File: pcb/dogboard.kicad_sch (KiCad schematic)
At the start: 41 parts, among them J1 USB-C / USB2.0, SW2 Action, SW3 Action, U1 RP2040, U3 8MB Flash, Y1 12 MHz

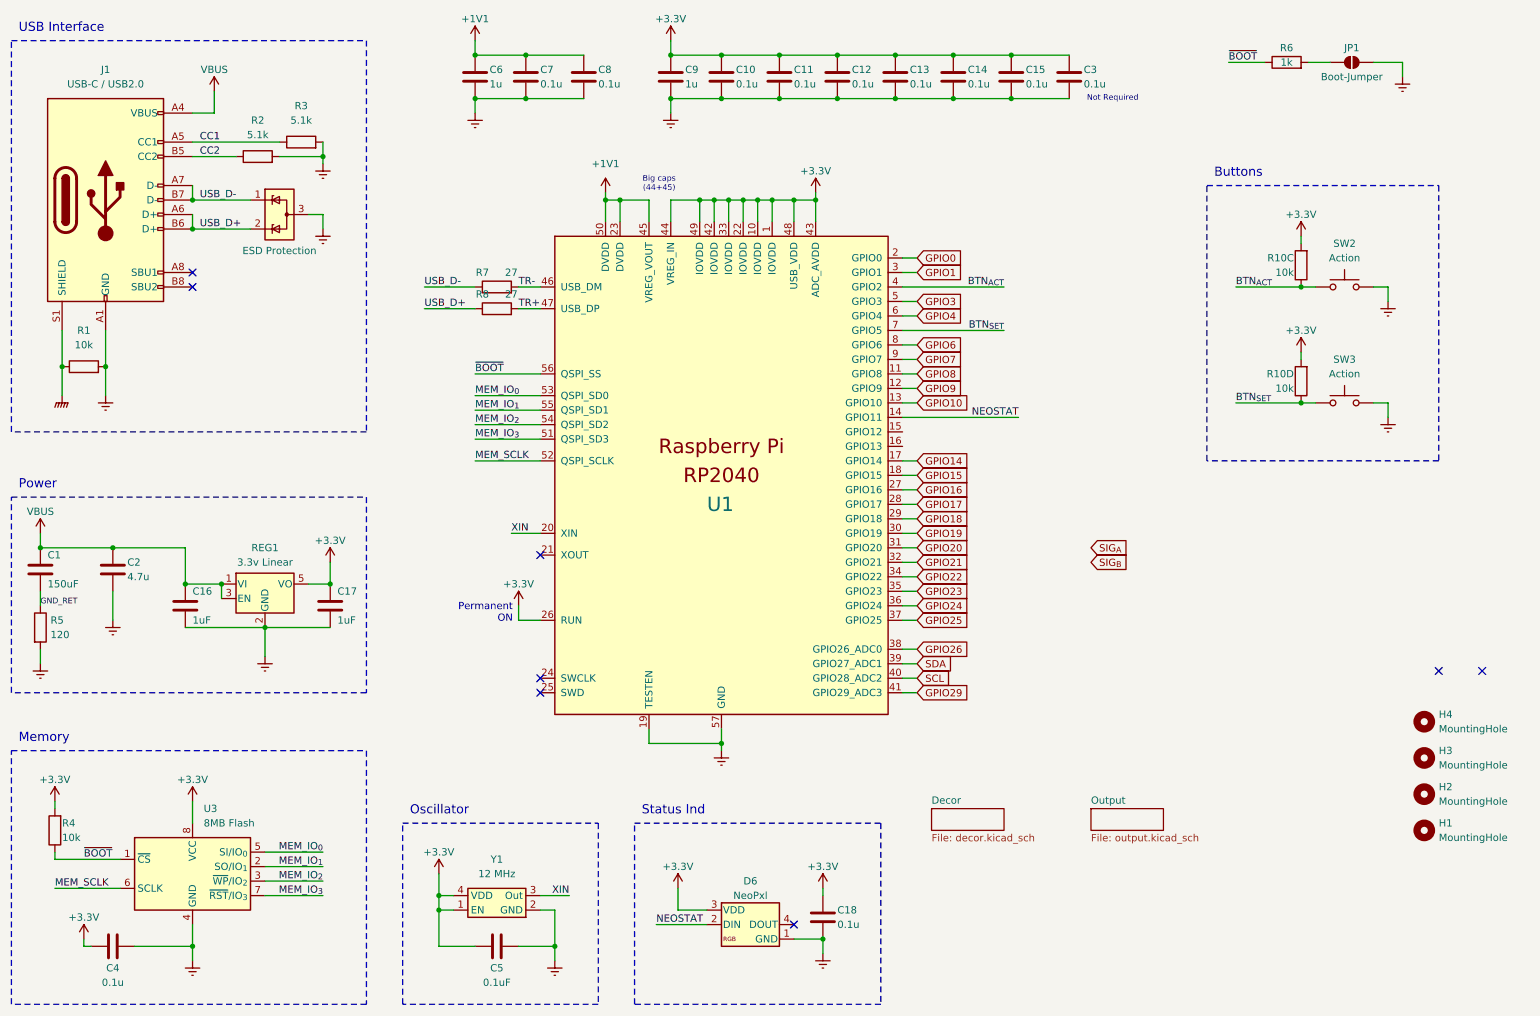
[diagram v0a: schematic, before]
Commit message: dogboard-2b4
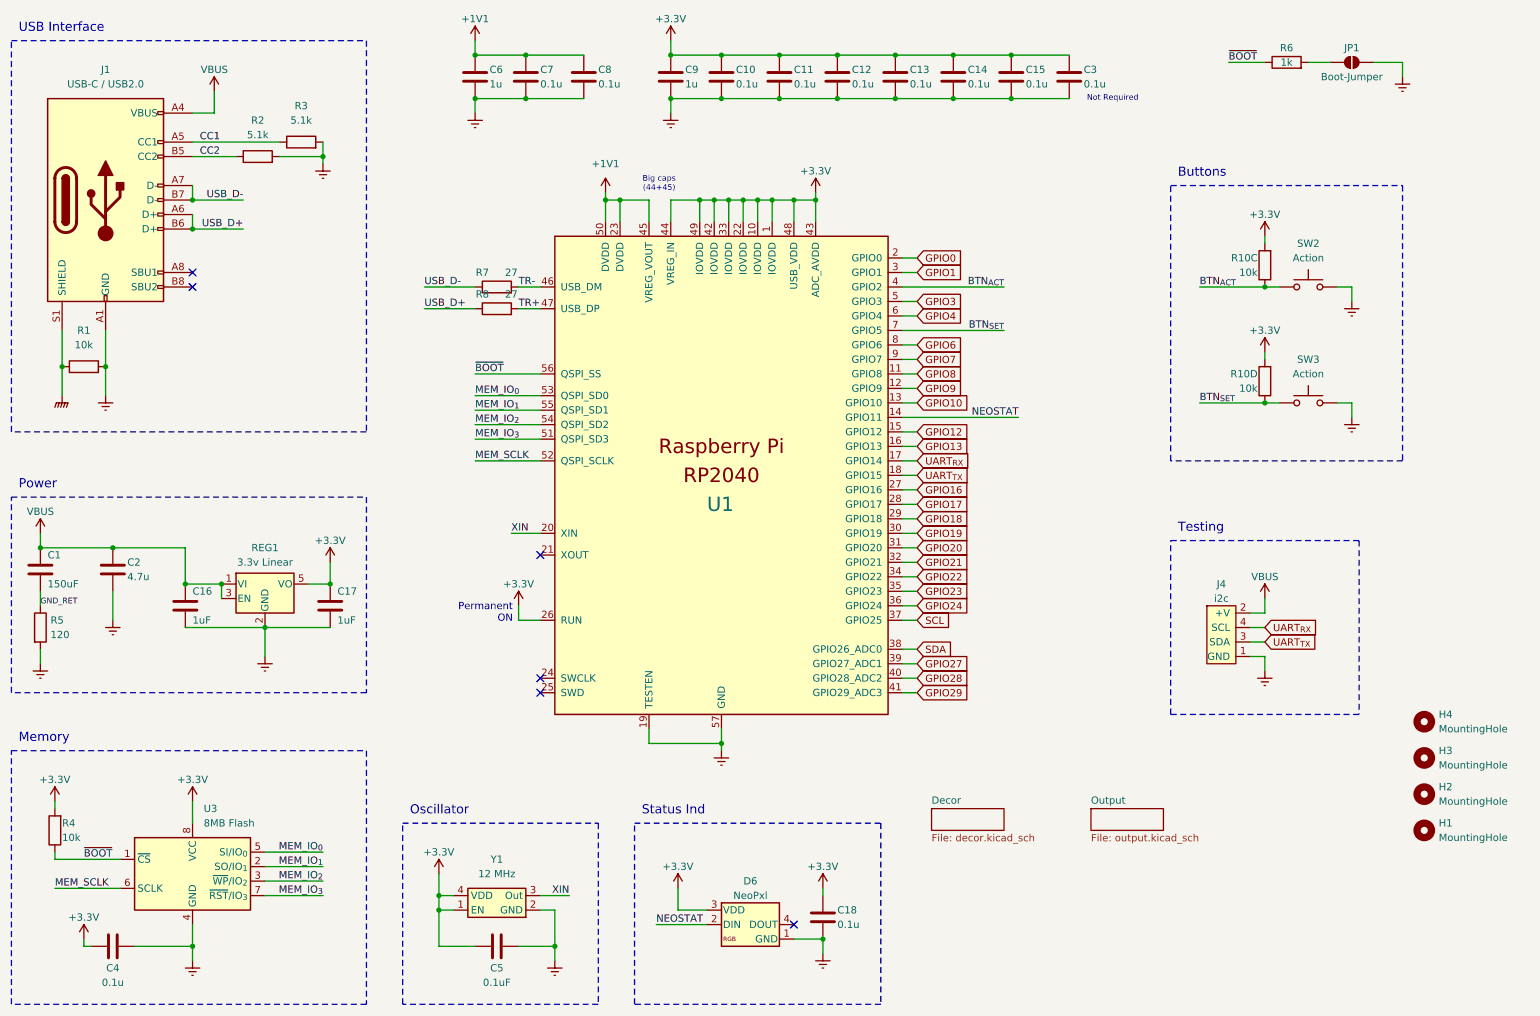
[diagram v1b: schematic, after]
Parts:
- removed D1: ESD Protection, _custom:tvs_USB2_SOT-723, symbol _custom:TVS_USB_ESD_Protection
- added J4: i2c, _custom:conn_1x04mp_JST_SH_Micro_P1.00mm_Horizontal, symbol _custom:i2c_connector
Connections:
- net GPIO25 is gone; now on net SCL: U1.37 (GPIO25)
- net GPIO26 is gone; now on net SDA: U1.38 (GPIO26_ADC0)
- net GNDREF: now also J4.1 (GND)
- net SCL: no longer U1.40 (GPIO28_ADC2)
- net SDA: no longer U1.39 (GPIO27_ADC1)
- net VBUS: now also J4.2 (+V)
- net GPIO12: now reaches U1.15 (GPIO12)
- net GPIO13: now reaches U1.16 (GPIO13)
- net GPIO14 renamed UART_{RX}
- net UART_{RX}: now also J4.4 (SCL)
- net GPIO15 renamed UART_{TX}
- net UART_{TX}: now also J4.3 (SDA)
- new net GPIO27: U1.39 (GPIO27_ADC1)
- new net GPIO28: U1.40 (GPIO28_ADC2)
- no-connect marks 8 -> 6
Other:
- note added: "Testing"
- moved on the sheet: R10C, R10D, SW2, SW3

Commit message: New board revision
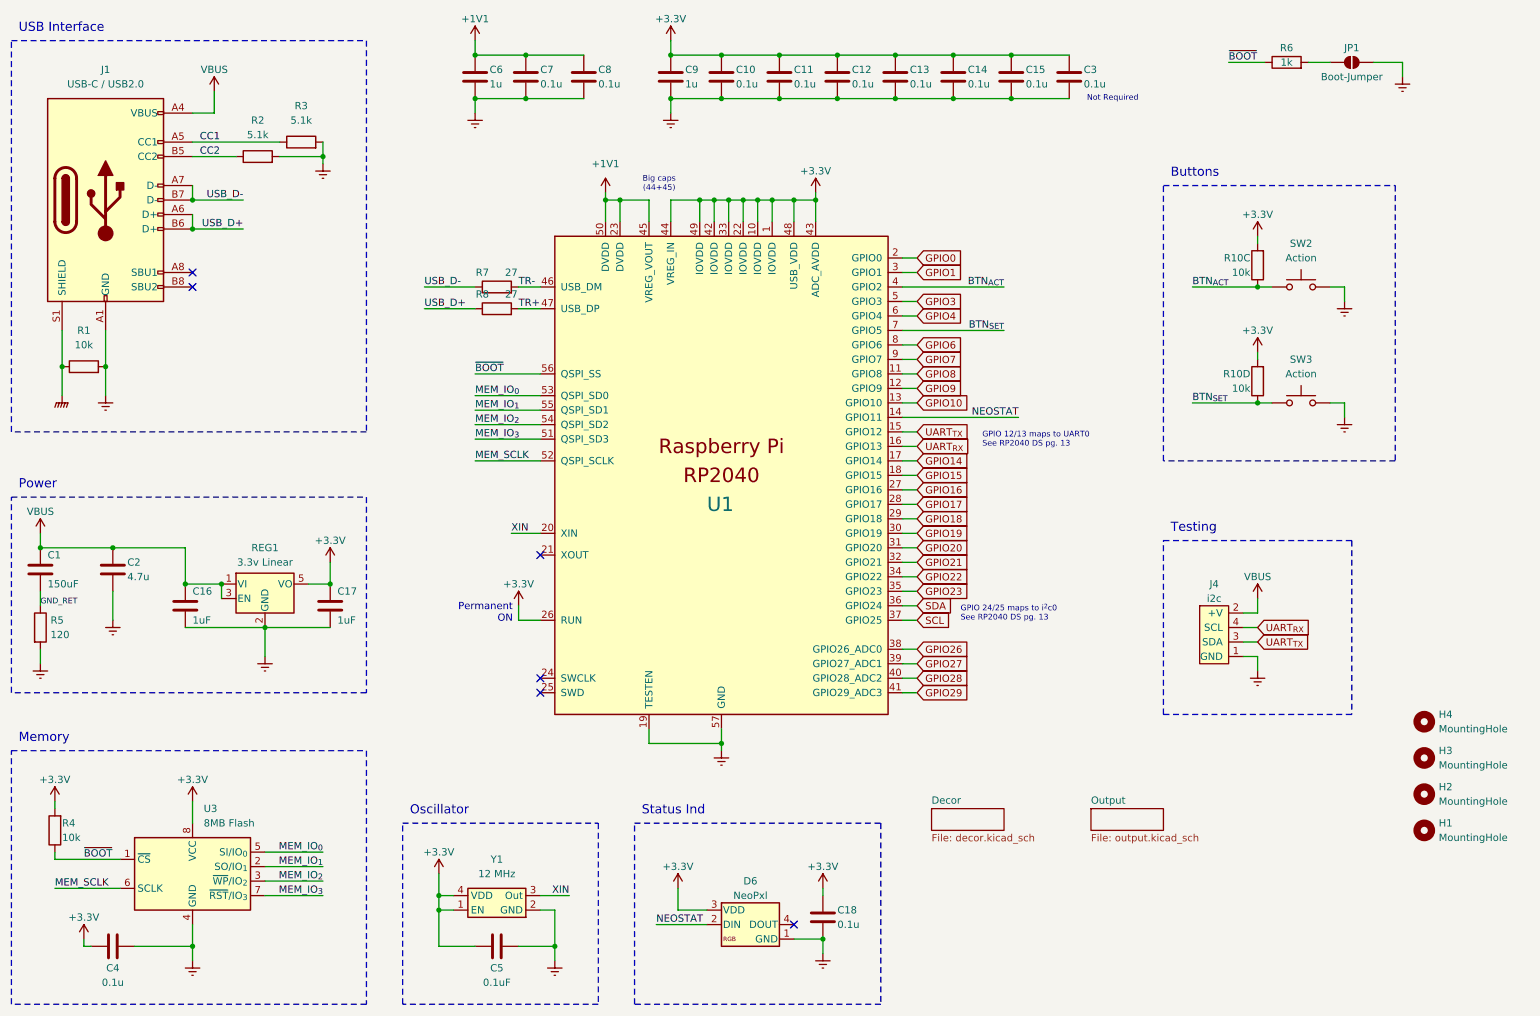
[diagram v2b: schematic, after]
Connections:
- net GPIO12 is gone; now on net UART_{TX}: U1.15 (GPIO12)
- net GPIO13 is gone; now on net UART_{RX}: U1.16 (GPIO13)
- net GPIO24 is gone; now on net SDA: U1.36 (GPIO24)
- net SDA: no longer U1.38 (GPIO26_ADC0)
- net UART_{RX}: no longer U1.17 (GPIO14)
- net UART_{TX}: no longer U1.18 (GPIO15)
- new net GPIO14: U1.17 (GPIO14)
- new net GPIO15: U1.18 (GPIO15)
- new net GPIO26: U1.38 (GPIO26_ADC0)
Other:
- note added: "GPIO 12/13 maps to UART0 See RP2040 DS pg. 13"
- note added: "GPIO 24/25 maps to i^{2}c0 See RP2040 DS pg. 13"
- moved on the sheet: J4, R10C, R10D, SW2, SW3
